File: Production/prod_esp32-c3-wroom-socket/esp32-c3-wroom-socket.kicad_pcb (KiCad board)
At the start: 2 copper layers, 30.5 x 25.4 mm, 10 parts, among them J3 USB-C_KUSBX-SL-CS1N14-B, SW1 SW_Push, U1 ESP32-C3-WROOM-02-N4, U2 AMS1117-3V3

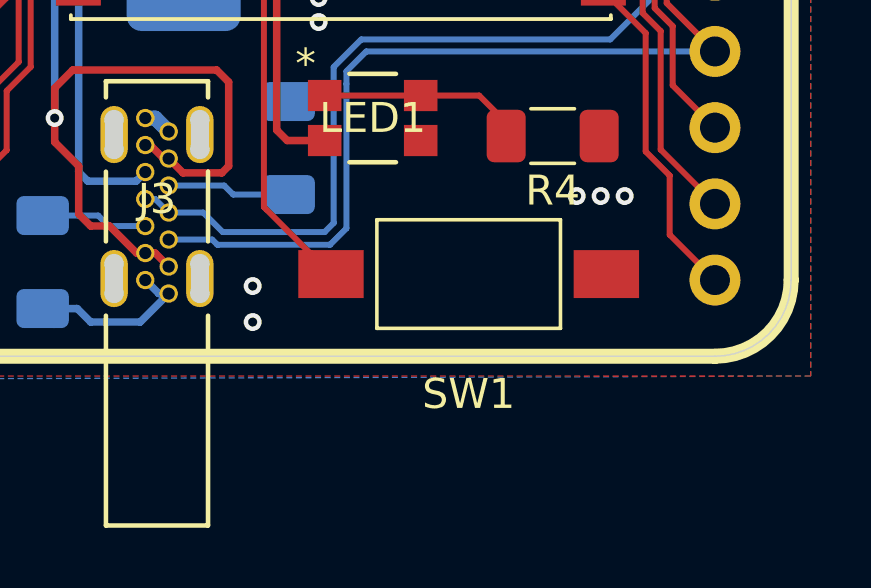
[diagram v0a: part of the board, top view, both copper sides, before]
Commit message: .
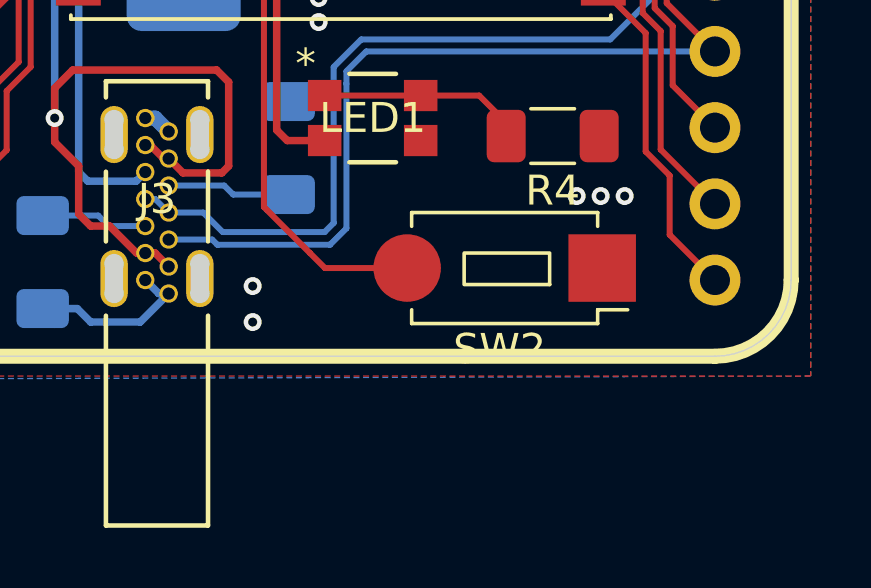
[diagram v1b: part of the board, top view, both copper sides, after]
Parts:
- removed SW1: SW_Push, Alexander Footprint Library:SW_SPST_6x3
- added SW2: SW_Push_SMD_6x3.5, Alexander Footprint Library:SW_PUSH_6x3.5mm, F.Cu at (165.7, 79.4)
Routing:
- net EN: track 35.6 -> 38.0 mm
